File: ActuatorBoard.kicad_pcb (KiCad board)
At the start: 2 copper layers, 75 x 89.5 mm, 79 parts, among them J1 Screw_Terminal_01x02, J11 Screw_Terminal_01x02, J12 Screw_Terminal_01x02, J13 Screw_Terminal_01x04, J2 Screw_Terminal_01x02, J3 Screw_Terminal_01x02, J4 Screw_Terminal_01x02, J5 Screw_Terminal_01x02, J7 Screw_Terminal_01x02, J8 Screw_Terminal_01x02, J9 Screw_Terminal_01x02, K1 SANYOU_SRD_Form_B, K2 SANYOU_SRD_Form_B, K3 SANYOU_SRD_Form_B, P1 CONN_01X03, P10 CONN_01X03, P11 CONN_01X03, P12 CONN_01X03, P13 CONN_01X02, P14 SERVO_+, P15 SERVO_-, P16 CONN_01X03, P17 CONN_01X05, P18 CONN_01X08, P19 CONN_01X05, P2 CAN_Conn, P20 CONN_01X08, P21 STEPPER_VCC, P22 CONN_01X05, P23 CONN_01X04, P3 CONN_01X03, P4 CONN_01X03, P5 CONN_01X03, P7 CONN_01X03, P8 CONN_01X03, Q1 BS170, Q2 BS170, Q3 BS170, Q5 IRLR024, U1 MCP2551-I-SN, U2 AT90CAN128-16AU, U3 ULN2003, U4 L7805, Y1 Crystal, Y2 Crystal

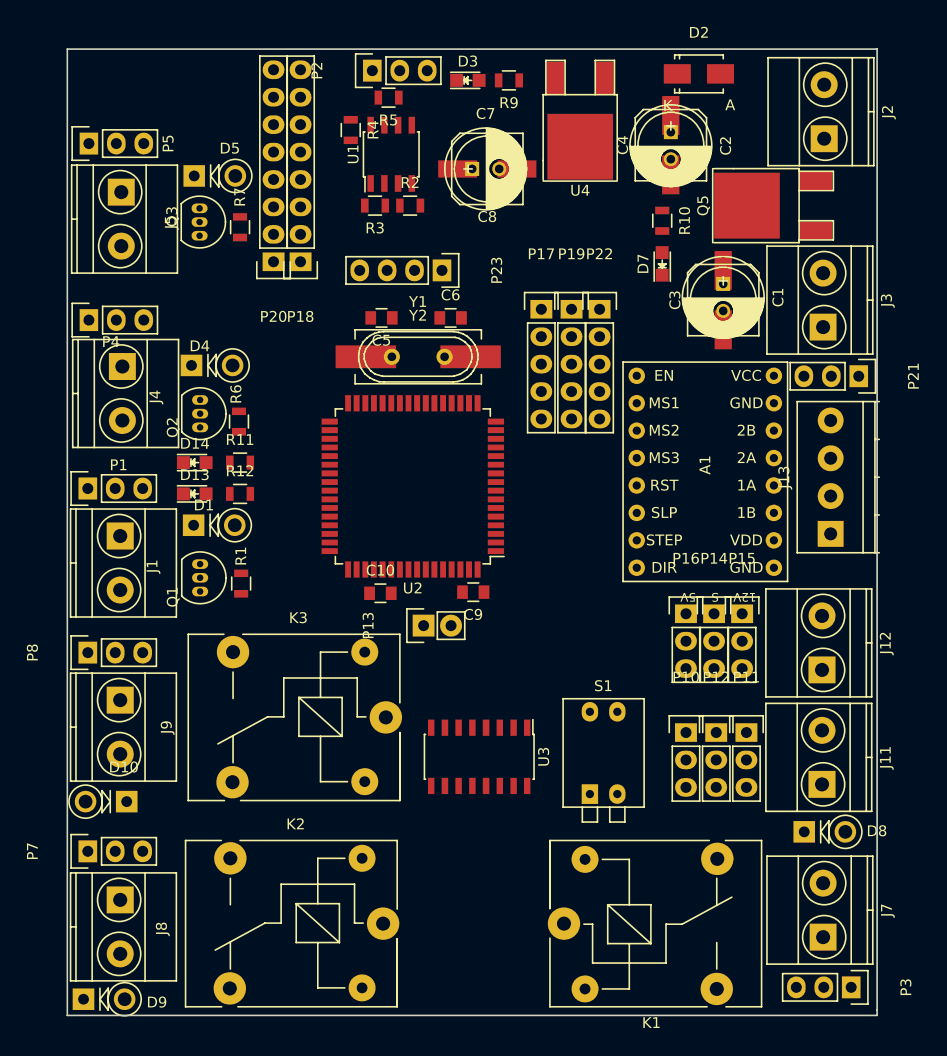
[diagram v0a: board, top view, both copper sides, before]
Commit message: Added output files
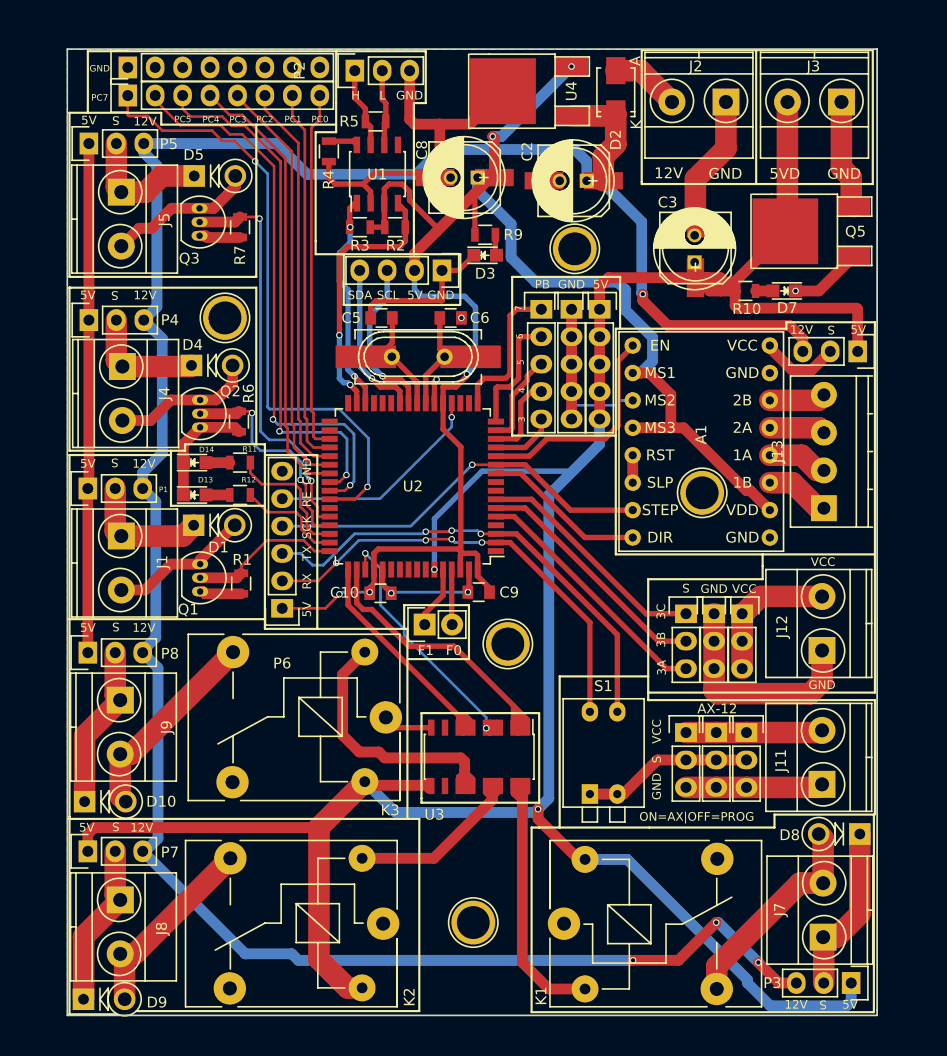
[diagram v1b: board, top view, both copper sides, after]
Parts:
- added P6: CONN_01X06, Pin_Headers:Pin_Header_Straight_1x06, F.Cu at (181.4, 76.3)
- added REF**: 1pin, Connect:1pin, F.Cu at (199.1, 105.4)
- added REF**: 1pin, Connect:1pin, F.Cu at (202.3, 79.6)
- added REF**: 1pin, Connect:1pin, F.Cu at (220.3, 65.6)
- added REF**: 1pin, Connect:1pin, F.Cu at (208.5, 43.0)
- added REF**: 1pin, Connect:1pin, F.Cu at (176.1, 49.4)
- moved P20 22.5 mm to (167.1, 26.2), turned to 90 degrees
- moved P18 22.2 mm to (167.1, 28.8), turned to 90 degrees
- moved J3 20.9 mm to (233.2, 29.4), turned to 180 degrees
- moved D3 16.3 mm to (200.2, 43.6)
- moved R9 14.5 mm to (200.2, 41.7), turned to 0 degrees
- moved D7 11.6 mm to (227.9, 46.9), turned to 180 degrees
- moved R10 10.1 mm to (224.3, 46.9), turned to 0 degrees
- moved J2 9.71 mm to (222.5, 29.4), turned to 180 degrees
- moved C4 9.59 mm to (208.4, 36.7), turned to 0 degrees
- moved C2 9.00 mm to (209.6, 36.7), turned to 180 degrees
- moved D2 7.89 mm to (212.3, 28.5), turned to 90 degrees
- moved C3 5.47 mm to (219.7, 42.9), turned to 270 degrees
- moved D8 5.15 mm to (234.9, 97.2), turned to 180 degrees
- moved Q5 4.27 mm to (234.3, 41.4)
- moved D10 3.90 mm to (163.1, 94.2), turned to 0 degrees
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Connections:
- P22 pad 1: +5V -> PF2
- P22 pad 2: +5V -> PF2
- P22 pad 3: +5V -> PF2
- P22 pad 4: +5V -> PF2
- P22 pad 5: +5V -> PF2
- R11 pad 2: Net-(R11-Pad2) -> D2
- R12 pad 2: Net-(R12-Pad2) -> D1
- S1 pad 3: RX0 -> TX0
- S1 pad 4: TX0 -> RX0
- U2 pad 10: STEP -> DIRECTION
- U2 pad 11: DIRECTION -> STEP
- U2 pad 20: (no net) -> RESET
- U2 pad 44: Net-(R11-Pad2) -> MINI_M3
- U2 pad 45: Net-(R12-Pad2) -> MINI_M2
- U2 pad 46: MINI_M3 -> D2
- U2 pad 47: MINI_M2 -> D1
- U3 pad 1: R1 -> R2
- U3 pad 13: R2_SIG -> R1_SIG
- U3 pad 14: R2_SIG -> R1_SIG
- U3 pad 15: R1_SIG -> R2_SIG
- U3 pad 16: R1_SIG -> R2_SIG
- U3 pad 2: R1 -> R2
- U3 pad 3: R2 -> R1
- U3 pad 4: R2 -> R1
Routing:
- net PF2: track 0.00 -> 292.9 mm, vias 0 -> 2
- net +12V: track 0.00 -> 226.9 mm, vias 0 -> 4
- net +5V: track 0.00 -> 158.3 mm, vias 0 -> 5
- net GND: track 0.00 -> 121.1 mm, vias 0 -> 5
- net PC7: track 0.00 -> 58.2 mm, vias 0 -> 2
- net PC6: track 0.00 -> 52.8 mm, vias 0 -> 2
- net PC5: track 0.00 -> 49.8 mm, vias 0 -> 2
- net TX0: track 0.00 -> 43.9 mm, vias 0 -> 3
- net RX0: track 0.00 -> 41.6 mm, vias 0 -> 4
- net PC4: track 0.00 -> 41.4 mm
- net PC3: track 0.00 -> 38.7 mm
- net MINI_M3: track 0.00 -> 37.8 mm, vias 0 -> 2
- net PC2: track 0.00 -> 36.8 mm
- net STEP: track 0.00 -> 36.6 mm, vias 0 -> 1
- net PC1: track 0.00 -> 34.9 mm
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- added copper zone on B.Cu, net GND
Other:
- board text added: "3"
- board text added: "3A"
- board text added: "3B"
- board text added: "3C"
- board text added: "4"
- board text added: "5"
- board text added: "5VD"
- board text added: "6"
- board text added: "7"
- board text added: "AX-12"
- board text added: "F0"
- board text added: "F1"
- board text added: "GND"
- board text added: "H"
- board text added: "L"
- board text added: "ON=AX|OFF=PROG"
- board text added: "PB"
- board text added: "PC0"
- board text added: "PC1"
- board text added: "PC2"
- board text added: "PC3"
- board text added: "PC4"
- board text added: "PC5"
- board text added: "PC7"
- board text added: "RE"
- board text added: "RX"
- board text added: "SCK"
- board text added: "SCL"
- board text added: "SDA"
- board text added: "TX"
- board text added: "VCC"
- board text added: "http://elektropioneer.co.rs/ https://github.com/Elektropioneer Actuator Board V1"
